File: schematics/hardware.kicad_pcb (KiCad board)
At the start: 2 copper layers, 10 parts, among them U1 CR2013-MI2120, U2 BMP280, U3 TXS0108EPW

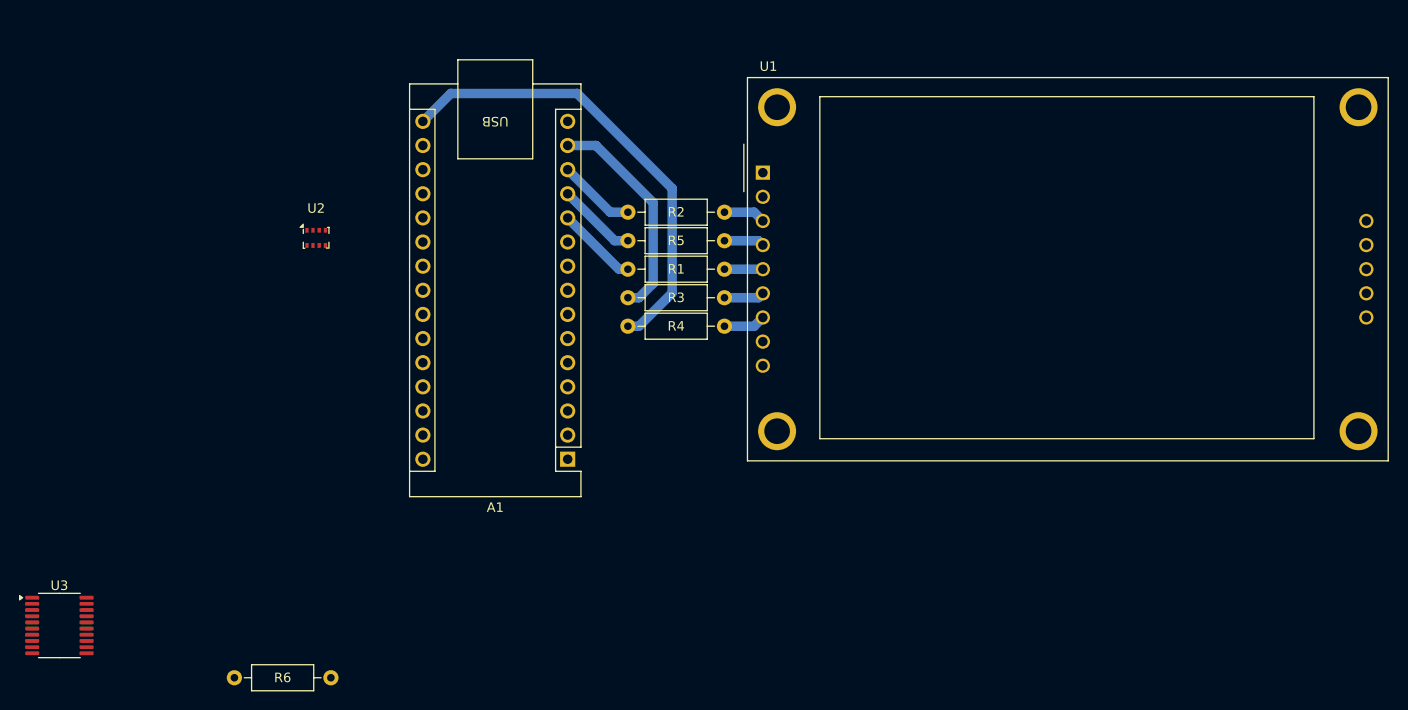
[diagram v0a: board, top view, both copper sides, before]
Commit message: pcbnew done
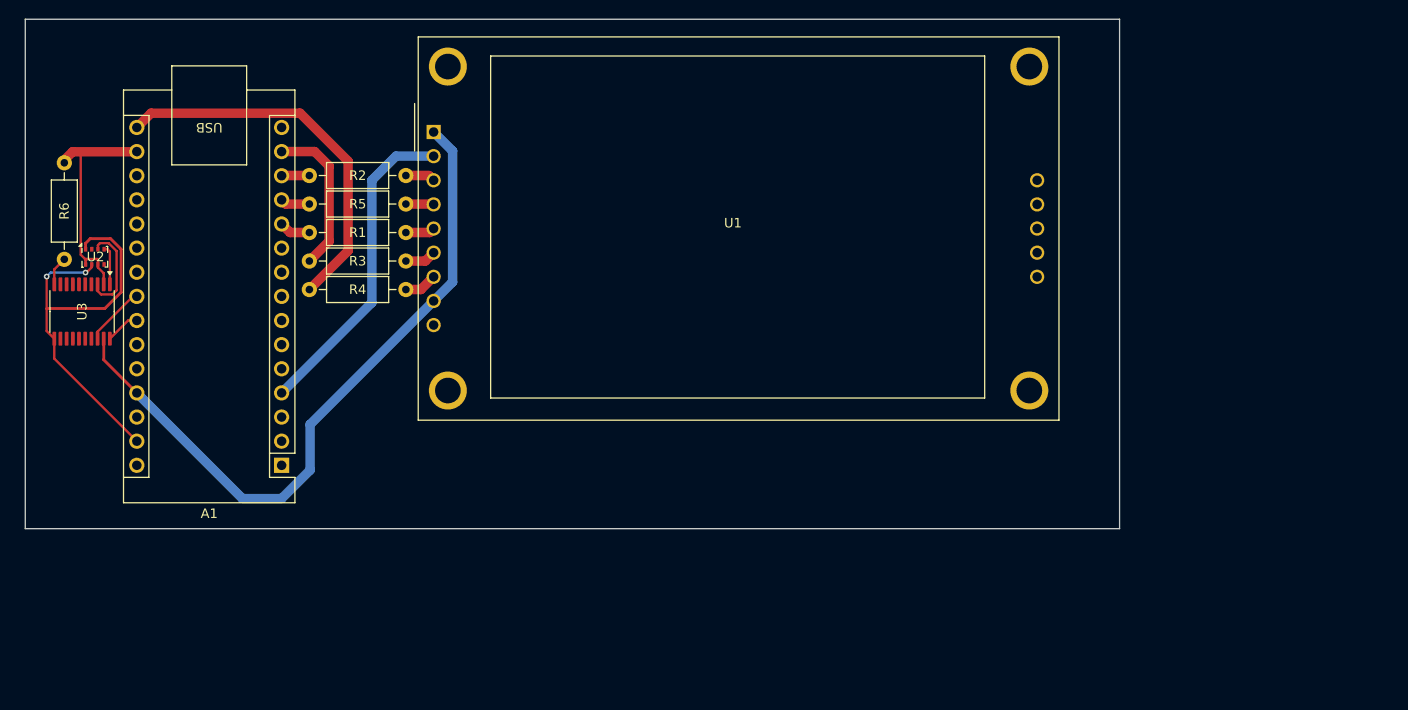
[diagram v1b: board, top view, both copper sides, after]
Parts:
- moved R6 47.5 mm to (19.0, 40.0), turned to 90 degrees
- moved U1 34.9 mm to (57.9, 26.6)
- moved R1 33.8 mm to (55.0, 37.1)
- moved R2 33.8 mm to (55.0, 31.1)
- moved R3 33.8 mm to (55.0, 40.1)
- moved R4 33.8 mm to (55.0, 43.1)
- moved R5 33.8 mm to (55.0, 34.1)
- moved U3 33.1 mm to (20.9, 45.5), turned to -90 degrees
- moved A1 30.1 mm to (41.9, 61.6)
- moved U2 23.4 mm to (22.2, 39.7)
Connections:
- A1 pad 23: /BMP_SDA -> /BMP_SDA_ARD
- A1 pad 24: /BMP_SCL -> /BMP_SCL_ARD
- U3 pad 18: /BMP_SDA -> /BMP_SDA_ARD
- U3 pad 20: /BMP_SCL -> /BMP_SCL_ARD
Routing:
- net GND: track 0.00 -> 78.7 mm, vias 0 -> 2
- net +5V: track 0.00 -> 73.9 mm
- net +3V3: track 0.00 -> 24.4 mm
- net /BMP_SDA: track 0.00 -> 9.99 mm
- net /TFT_SCK: track 48.7 -> 40.1 mm
- net /TFT_MOSI: track 23.3 -> 16.5 mm
- net /BMP_SDA_ARD: track 0.00 -> 5.99 mm
- net /TFT_RESET: track 8.39 -> 3.10 mm
- net /TFT_DC: track 8.58 -> 3.29 mm
- net /TFT_CS: track 8.20 -> 2.93 mm
- net /BMP_SCL: track 0.00 -> 4.16 mm
- net /BMP_SCL_ARD: track 0.00 -> 3.63 mm
- net Net-(U3-OE): track 0.00 -> 3.07 mm
- net Net-(U1-~{CS}): track 4.42 -> 3.13 mm
- net Net-(U1-RESET): track 4.23 -> 2.94 mm
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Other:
- board outline added: 115.2 x 53.6 mm
